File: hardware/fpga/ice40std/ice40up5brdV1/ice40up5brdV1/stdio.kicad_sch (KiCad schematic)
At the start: 17 parts, among them J1 Conn_01x20_Male, J2 Conn_01x20_Female, SW1 SW_Push, SW2 SW_Push, SW3 SW_Push

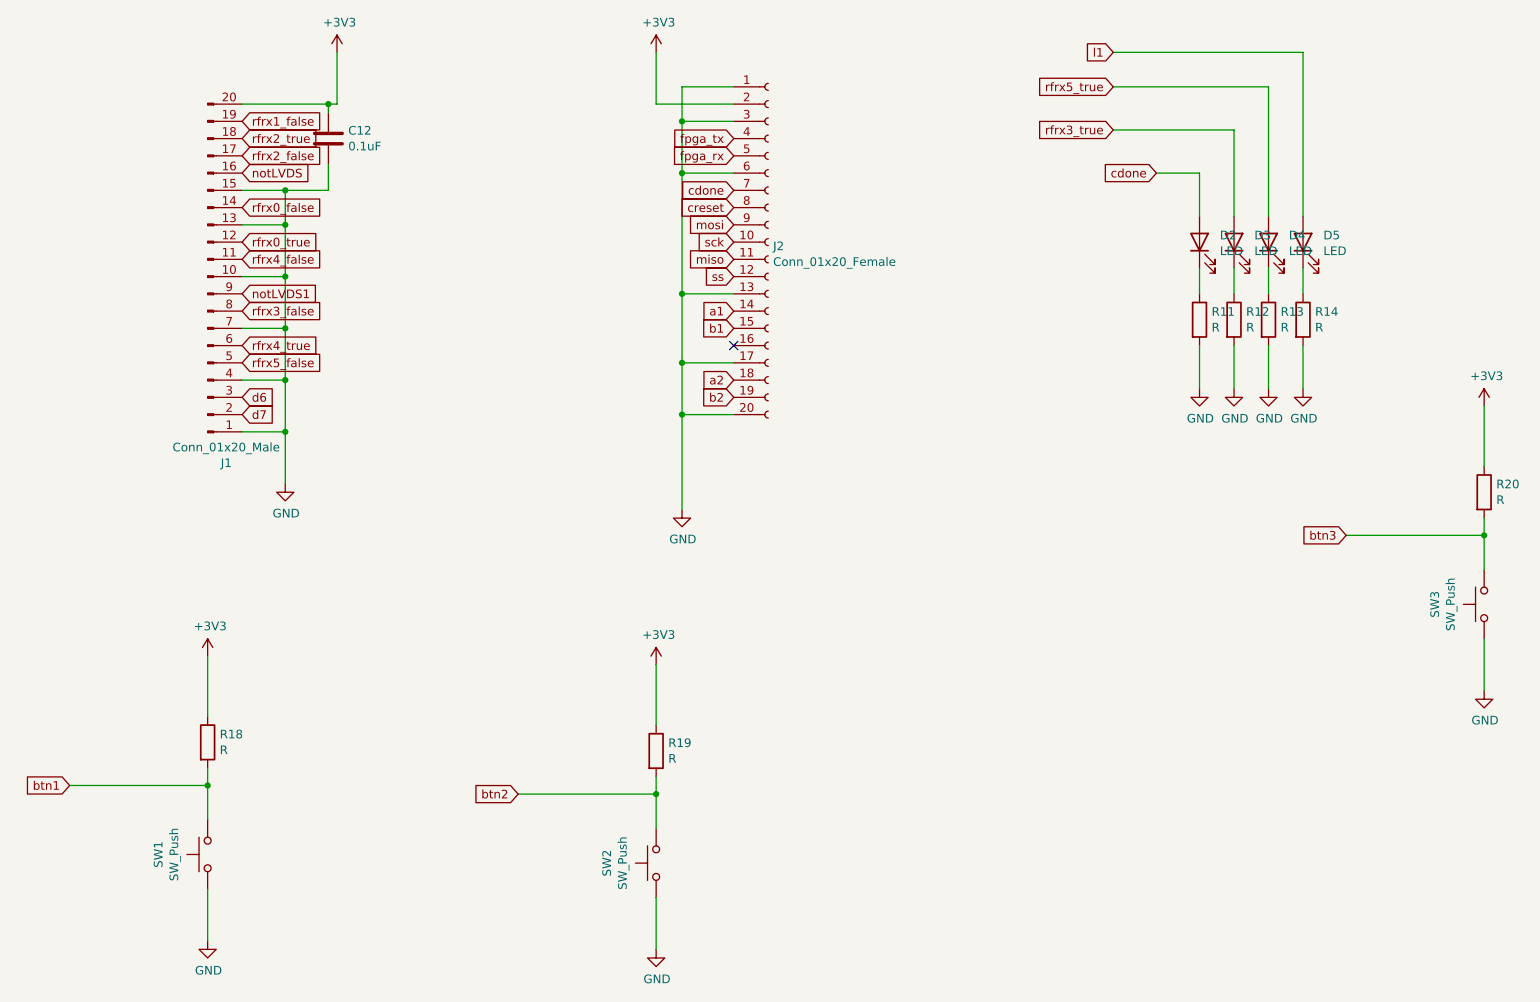
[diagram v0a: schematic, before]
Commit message: pwm / lvds power / filters
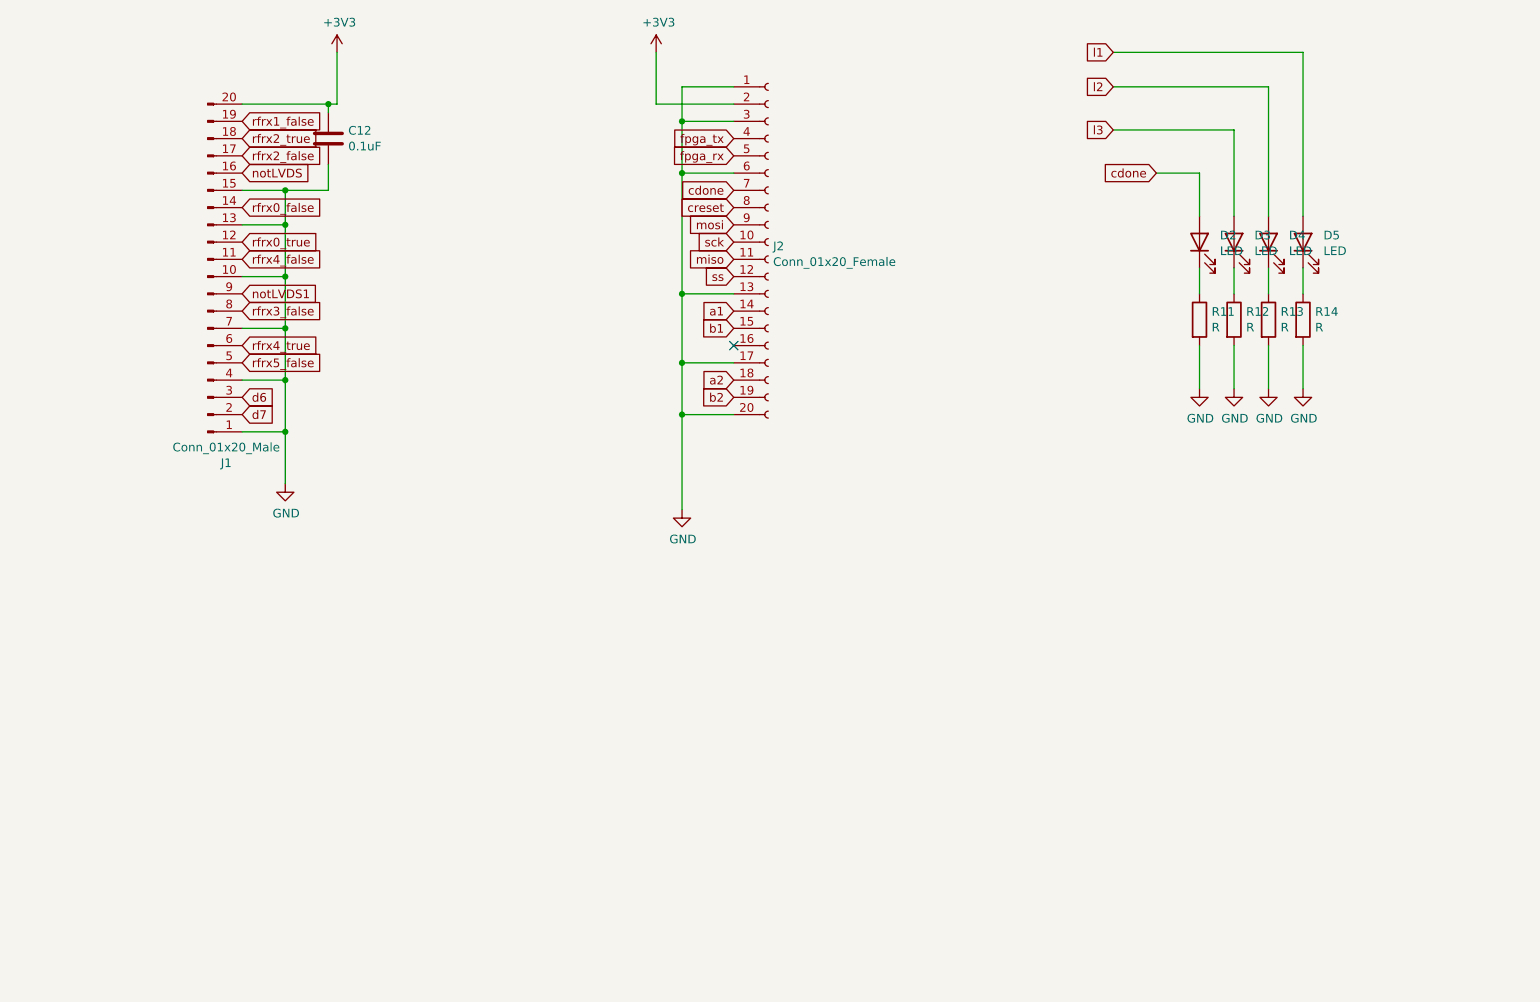
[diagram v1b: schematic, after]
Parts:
- removed R18, R19, R20: R, Resistor_SMD:R_0402_1005Metric, symbol Device:R
- removed SW1, SW2, SW3: SW_Push, Button_Switch_THT:SW_PUSH_6mm_H8mm, symbol Switch:SW_Push
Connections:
- net rfrx3_true renamed l3
- net rfrx5_true renamed l2

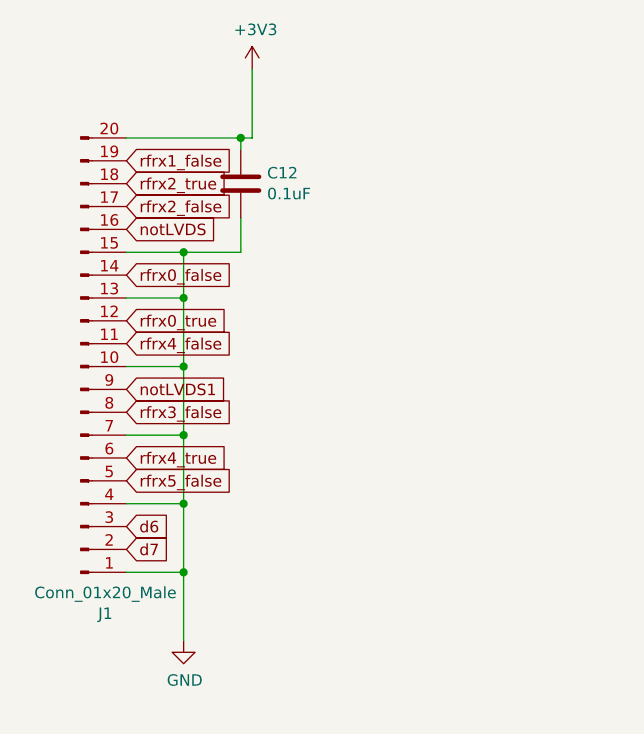
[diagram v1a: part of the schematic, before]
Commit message: pwm / lvds power / filters
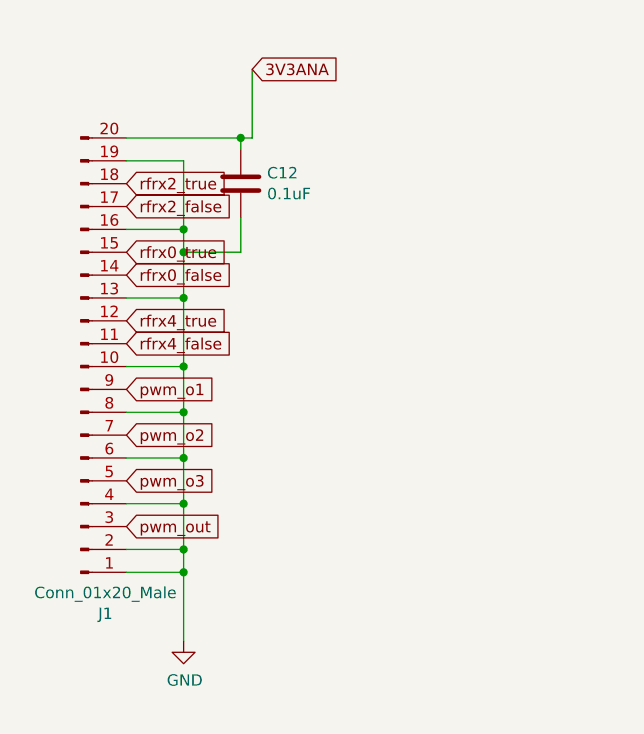
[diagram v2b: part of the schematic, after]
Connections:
- net d7 is gone; now on net GND: J1.2 (Pin_2)
- net notLVDS is gone; now on net GND: J1.16 (Pin_16)
- net rfrx1_false is gone; now on net GND: J1.19 (Pin_19)
- net rfrx3_false is gone; now on net GND: J1.8 (Pin_8)
- net +3V3: no longer C12.1, J1.20 (Pin_20)
- net GND: now also J1.6 (Pin_6); no longer J1.15 (Pin_15), J1.7 (Pin_7)
- net rfrx0_true: now also J1.15 (Pin_15); no longer J1.12 (Pin_12)
- net rfrx4_true: now also J1.12 (Pin_12); no longer J1.6 (Pin_6)
- net d6 renamed pwm_out
- net notLVDS1 renamed pwm_o1
- net rfrx5_false renamed pwm_o3
- new net 3V3ANA: C12.1, J1.20 (Pin_20)
- new net pwm_o2: J1.7 (Pin_7)
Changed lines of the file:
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@@
   (junction (at 73.66 102.87) (diameter 0) (color 0 0 0 0)
   )
+  (junction (at 73.66 100.33) (diameter 0) (color 0 0 0 0)
+  )
   (junction (at 132.08 64.77) (diameter 0) (color 0 0 0 0)
   )
   (junction (at 132.08 92.71) (diameter 0) (color 0 0 0 0)
   )
-  (junction (at 73.66 87.63) (diameter 0) (color 0 0 0 0)
+  (junction (at 73.66 85.09) (diameter 0) (color 0 0 0 0)
   )
   (junction (at 132.08 100.33) (diameter 0) (color 0 0 0 0)
@@
   (junction (at 73.66 67.31) (diameter 0) (color 0 0 0 0)
   )
+  (junction (at 73.66 64.77) (diameter 0) (color 0 0 0 0)
+  )
   (junction (at 80.01 54.61) (diameter 0) (color 0 0 0 0)
   )
   (junction (at 73.66 95.25) (diameter 0) (color 0 0 0 0)
+  )
+  (junction (at 73.66 90.17) (diameter 0) (color 0 0 0 0)
   )
   (junction (at 73.66 72.39) (diameter 0) (color 0 0 0 0)
@@
     (stroke (width 0) (type default) (color 0 0 0 0))
   )
+  (wire (pts (xy 67.31 57.15) (xy 73.66 57.15))
+    (stroke (width 0) (type default) (color 0 0 0 0))
+  )
   (wire (pts (xy 218.44 90.17) (xy 218.44 96.52))
     (stroke (width 0) (type default) (color 0 0 0 0))
@@
     (stroke (width 0) (type default) (color 0 0 0 0))
   )
-  (wire (pts (xy 73.66 95.25) (xy 73.66 102.87))
+  (wire (pts (xy 73.66 95.25) (xy 73.66 100.33))
+    (stroke (width 0) (type default) (color 0 0 0 0))
+  )
+  (wire (pts (xy 67.31 90.17) (xy 73.66 90.17))
     (stroke (width 0) (type default) (color 0 0 0 0))
   )
@@
     (stroke (width 0) (type default) (color 0 0 0 0))
   )
-  (wire (pts (xy 73.66 95.25) (xy 73.66 87.63))
-    (stroke (width 0) (type default) (color 0 0 0 0))
-  )
   (wire (pts (xy 73.66 67.31) (xy 80.01 67.31))
     (stroke (width 0) (type default) (color 0 0 0 0))
   )
-  (wire (pts (xy 73.66 80.01) (xy 73.66 87.63))
+  (wire (pts (xy 73.66 80.01) (xy 73.66 85.09))
     (stroke (width 0) (type default) (color 0 0 0 0))
   )
@@
     (stroke (width 0) (type default) (color 0 0 0 0))
   )
+  (wire (pts (xy 73.66 90.17) (xy 73.66 95.25))
+    (stroke (width 0) (type default) (color 0 0 0 0))
+  )
   (wire (pts (xy 195.58 58.42) (xy 213.36 58.42))
     (stroke (width 0) (type default) (color 0 0 0 0))
@@
     (stroke (width 0) (type default) (color 0 0 0 0))
   )
+  (wire (pts (xy 67.31 64.77) (xy 73.66 64.77))
+    (stroke (width 0) (type default) (color 0 0 0 0))
+  )
+  (wire (pts (xy 73.66 100.33) (xy 73.66 102.87))
+    (stroke (width 0) (type default) (color 0 0 0 0))
+  )
   (wire (pts (xy 132.08 82.55) (xy 132.08 92.71))
     (stroke (width 0) (type default) (color 0 0 0 0))
@@
     (stroke (width 0) (type default) (color 0 0 0 0))
   )
-  (wire (pts (xy 67.31 67.31) (xy 73.66 67.31))
+  (wire (pts (xy 67.31 100.33) (xy 73.66 100.33))
+    (stroke (width 0) (type default) (color 0 0 0 0))
+  )
+  (wire (pts (xy 73.66 64.77) (xy 73.66 67.31))
     (stroke (width 0) (type default) (color 0 0 0 0))
   )
@@
     (stroke (width 0) (type default) (color 0 0 0 0))
   )
+  (wire (pts (xy 73.66 85.09) (xy 73.66 90.17))
+    (stroke (width 0) (type default) (color 0 0 0 0))
+  )
   (wire (pts (xy 67.31 72.39) (xy 73.66 72.39))
     (stroke (width 0) (type default) (color 0 0 0 0))
@@
     (stroke (width 0) (type default) (color 0 0 0 0))
   )
-  (wire (pts (xy 73.66 87.63) (xy 67.31 87.63))
+  (wire (pts (xy 67.31 85.09) (xy 73.66 85.09))
+    (stroke (width 0) (type default) (color 0 0 0 0))
+  )
+  (wire (pts (xy 73.66 57.15) (xy 73.66 64.77))
     (stroke (width 0) (type default) (color 0 0 0 0))
   )
@@
   (wire (pts (xy 139.7 52.07) (xy 132.08 52.07))
     (stroke (width 0) (type default) (color 0 0 0 0))
-  )
-  (global_label "rfrx5_false" (shape input) (at 67.31 92.71 0) (fields_autoplaced)
-    (effects (font (size 1.27 1.27)) (justify left))
-    (property "Intersheet References" "${INTERSHEET_REFS}" (id 0) (at 0 0 0)
-      (effects (font (size 1.27 1.27)) hide)
-    )
   )
   (global_label "b2" (shape input) (at 139.7 97.79 180) (fields_autoplaced)
@@
     )
   )
+  (global_label "pwm_o1" (shape input) (at 67.31 82.55 0) (fields_autoplaced)
+    (effects (font (size 1.27 1.27)) (justify left))
+    (property "Intersheet References" "${INTERSHEET_REFS}" (id 0) (at 77.1332 82.6294 0)
+      (effects (font (size 1.27 1.27)) (justify left) hide)
+    )
+  )
   (global_label "b1" (shape input) (at 139.7 87.63 180) (fields_autoplaced)
     (effects (font (size 1.27 1.27)) (justify right))
@@
     )
   )
+  (global_label "pwm_o2" (shape input) (at 67.31 87.63 0) (fields_autoplaced)
+    (effects (font (size 1.27 1.27)) (justify left))
+    (property "Intersheet References" "${INTERSHEET_REFS}" (id 0) (at 77.1332 87.7094 0)
+      (effects (font (size 1.27 1.27)) (justify left) hide)
+    )
+  )
   (global_label "miso" (shape input) (at 139.7 77.47 180) (fields_autoplaced)
     (effects (font (size 1.27 1.27)) (justify right))
@@
     )
   )
-  (global_label "rfrx3_false" (shape input) (at 67.31 85.09 0) (fields_autoplaced)
-    (effects (font (size 1.27 1.27)) (justify left))
-    (property "Intersheet References" "${INTERSHEET_REFS}" (id 0) (at 0 0 0)
-      (effects (font (size 1.27 1.27)) hide)
-    )
-  )
-  (global_label "notLVDS" (shape input) (at 67.31 64.77 0) (fields_autoplaced)
-    (effects (font (size 1.27 1.27)) (justify left))
-    (property "Intersheet References" "${INTERSHEET_REFS}" (id 0) (at 0 0 0)
-      (effects (font (size 1.27 1.27)) hide)
-    )
-  )
   (global_label "fpga_rx" (shape input) (at 139.7 62.23 180) (fields_autoplaced)
     (effects (font (size 1.27 1.27)) (justify right))
@@
     )
   )
-  (global_label "rfrx1_false" (shape input) (at 67.31 57.15 0) (fields_autoplaced)
-    (effects (font (size 1.27 1.27)) (justify left))
-    (property "Intersheet References" "${INTERSHEET_REFS}" (id 0) (at 0 0 0)
-      (effects (font (size 1.27 1.27)) hide)
-    )
-  )
-  (global_label "rfrx0_true" (shape input) (at 67.31 74.93 0) (fields_autoplaced)
-    (effects (font (size 1.27 1.27)) (justify left))
-    (property "Intersheet References" "${INTERSHEET_REFS}" (id 0) (at 0 0 0)
+  (global_label "3V3ANA" (shape input) (at 81.28 46.99 0) (fields_autoplaced)
+    (effects (font (size 1.27 1.27)) (justify left))
+    (property "Intersheet References" "${INTERSHEET_REFS}" (id 0) (at 90.6194 46.9106 0)
+      (effects (font (size 1.27 1.27)) (justify left) hide)
+    )
+  )
+  (global_label "rfrx0_true" (shape input) (at 67.31 67.31 0) (fields_autoplaced)
+    (effects (font (size 1.27 1.27)) (justify left))
+    (property "Intersheet References" "${INTERSHEET_REFS}" (id 0) (at 0 -7.62 0)
       (effects (font (size 1.27 1.27)) hide)
     )
@@
     )
   )
+  (global_label "pwm_o3" (shape input) (at 67.31 92.71 0) (fields_autoplaced)
+    (effects (font (size 1.27 1.27)) (justify left))
+    (property "Intersheet References" "${INTERSHEET_REFS}" (id 0) (at 77.1332 92.7894 0)
+      (effects (font (size 1.27 1.27)) (justify left) hide)
+    )
+  )
   (global_label "a1" (shape input) (at 139.7 85.09 180) (fields_autoplaced)
     (effects (font (size 1.27 1.27)) (justify right))
@@
     )
   )
+  (global_label "pwm_out" (shape input) (at 67.31 97.79 0) (fields_autoplaced)
+    (effects (font (size 1.27 1.27)) (justify left))
+    (property "Intersheet References" "${INTERSHEET_REFS}" (id 0) (at 77.7985 97.8694 0)
+      (effects (font (size 1.27 1.27)) (justify left) hide)
+    )
+  )
   (global_label "rfrx2_true" (shape input) (at 67.31 59.69 0) (fields_autoplaced)
     (effects (font (size 1.27 1.27)) (justify left))
@@
     )
   )
-  (global_label "d7" (shape input) (at 67.31 100.33 0) (fields_autoplaced)
-    (effects (font (size 1.27 1.27)) (justify left))
-    (property "Intersheet References" "${INTERSHEET_REFS}" (id 0) (at 0 0 0)
-      (effects (font (size 1.27 1.27)) hide)
-    )
-  )
-  (global_label "rfrx4_true" (shape input) (at 67.31 90.17 0) (fields_autoplaced)
-    (effects (font (size 1.27 1.27)) (justify left))
-    (property "Intersheet References" "${INTERSHEET_REFS}" (id 0) (at 0 0 0)
-      (effects (font (size 1.27 1.27)) hide)
-    )
-  )
   (global_label "mosi" (shape input) (at 139.7 72.39 180) (fields_autoplaced)
     (effects (font (size 1.27 1.27)) (justify right))
@@
     )
   )
-  (global_label "d6" (shape input) (at 67.31 97.79 0) (fields_autoplaced)
-    (effects (font (size 1.27 1.27)) (justify left))
-    (property "Intersheet References" "${INTERSHEET_REFS}" (id 0) (at 0 0 0)
+  (global_label "rfrx4_true" (shape input) (at 67.31 74.93 0) (fields_autoplaced)
+    (effects (font (size 1.27 1.27)) (justify left))
+    (property "Intersheet References" "${INTERSHEET_REFS}" (id 0) (at 0 -15.24 0)
       (effects (font (size 1.27 1.27)) hide)
     )
@@
     (property "Intersheet References" "${INTERSHEET_REFS}" (id 0) (at 191.381 58.3406 0)
       (effects (font (size 1.27 1.27)) (justify right) hide)
-    )
-  )
-  (global_label "notLVDS1" (shape input) (at 67.31 82.55 0) (fields_autoplaced)
-    (effects (font (size 1.27 1.27)) (justify left))
-    (property "Intersheet References" "${INTERSHEET_REFS}" (id 0) (at 0 0 0)
-      (effects (font (size 1.27 1.27)) hide)
     )
   )
@@
       (effects (font (size 1.27 1.27)) hide)
     )
-    (pin "1")
-  )
-  (symbol (lib_id "power:+3V3") (at 81.28 46.99 0) (unit 1)
-    (in_bom yes) (on_board yes)
-    (property "Reference" "#PWR034" (id 0) (at 81.28 50.8 0)
-      (effects (font (size 1.27 1.27)) hide)
-    )
-    (property "Value" "+3V3" (id 1) (at 81.661 42.5958 0))
-    (property "Footprint" "" (id 2) (at 81.28 46.99 0)
-      (effects (font (size 1.27 1.27)) hide)
-    )
-    (property "Datasheet" "" (id 3) (at 81.28 46.99 0)
-      (effects (font (size 1.27 1.27)) hide)
-    )

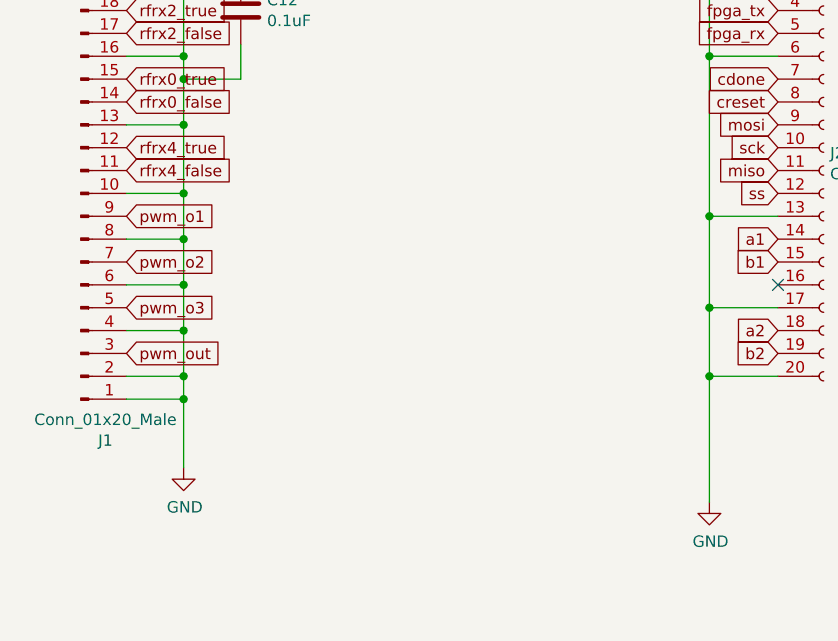
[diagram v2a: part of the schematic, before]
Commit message: pwm / lvds power / filters
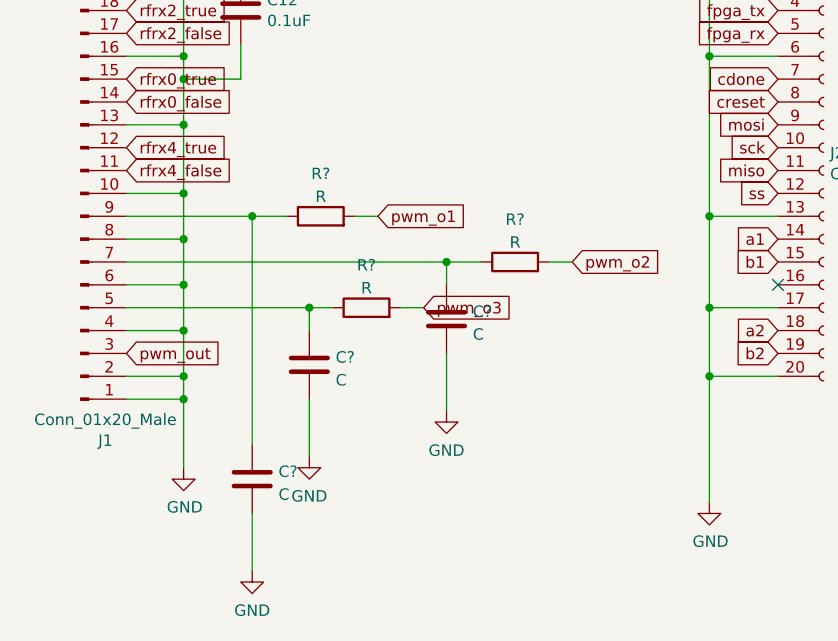
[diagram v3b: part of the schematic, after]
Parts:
- added C? (x3): C, symbol Device:C
- added R? (x3): R, symbol Device:R
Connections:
- net GND: now also C?.2, C?.2, C?.2
- net pwm_o1: now also R?.2; no longer J1.9 (Pin_9)
- net pwm_o2: now also R?.2; no longer J1.7 (Pin_7)
- net pwm_o3: now also R?.2; no longer J1.5 (Pin_5)
- new net: C?.1, J1.5 (Pin_5), R?.1
- new net: C?.1, J1.7 (Pin_7), R?.1
- new net: C?.1, J1.9 (Pin_9), R?.1
